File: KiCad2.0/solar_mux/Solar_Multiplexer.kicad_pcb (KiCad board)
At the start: 2 copper layers, 229.4 x 213.5 mm, 34 parts, among them J1 Conn_01x14, J2 Conn_02x06_Odd_Even, J3 Conn_02x06_Odd_Even, U1 ASSR-1611, U10 ASSR-1611, U11 ASSR-1611, U12 ASSR-1611, U13 ASSR-1611, U14 ASSR-1611, U15 ASSR-1611, U16 ASSR-1611, U17 ASSR-1611, U2 ASSR-1611, U20 ASSR-1611, U21 ASSR-1611, U22 MCP23S17, U3 ASSR-1611, U4 ASSR-1611, U5 ASSR-1611, U6 ASSR-1611, U7 ASSR-1611

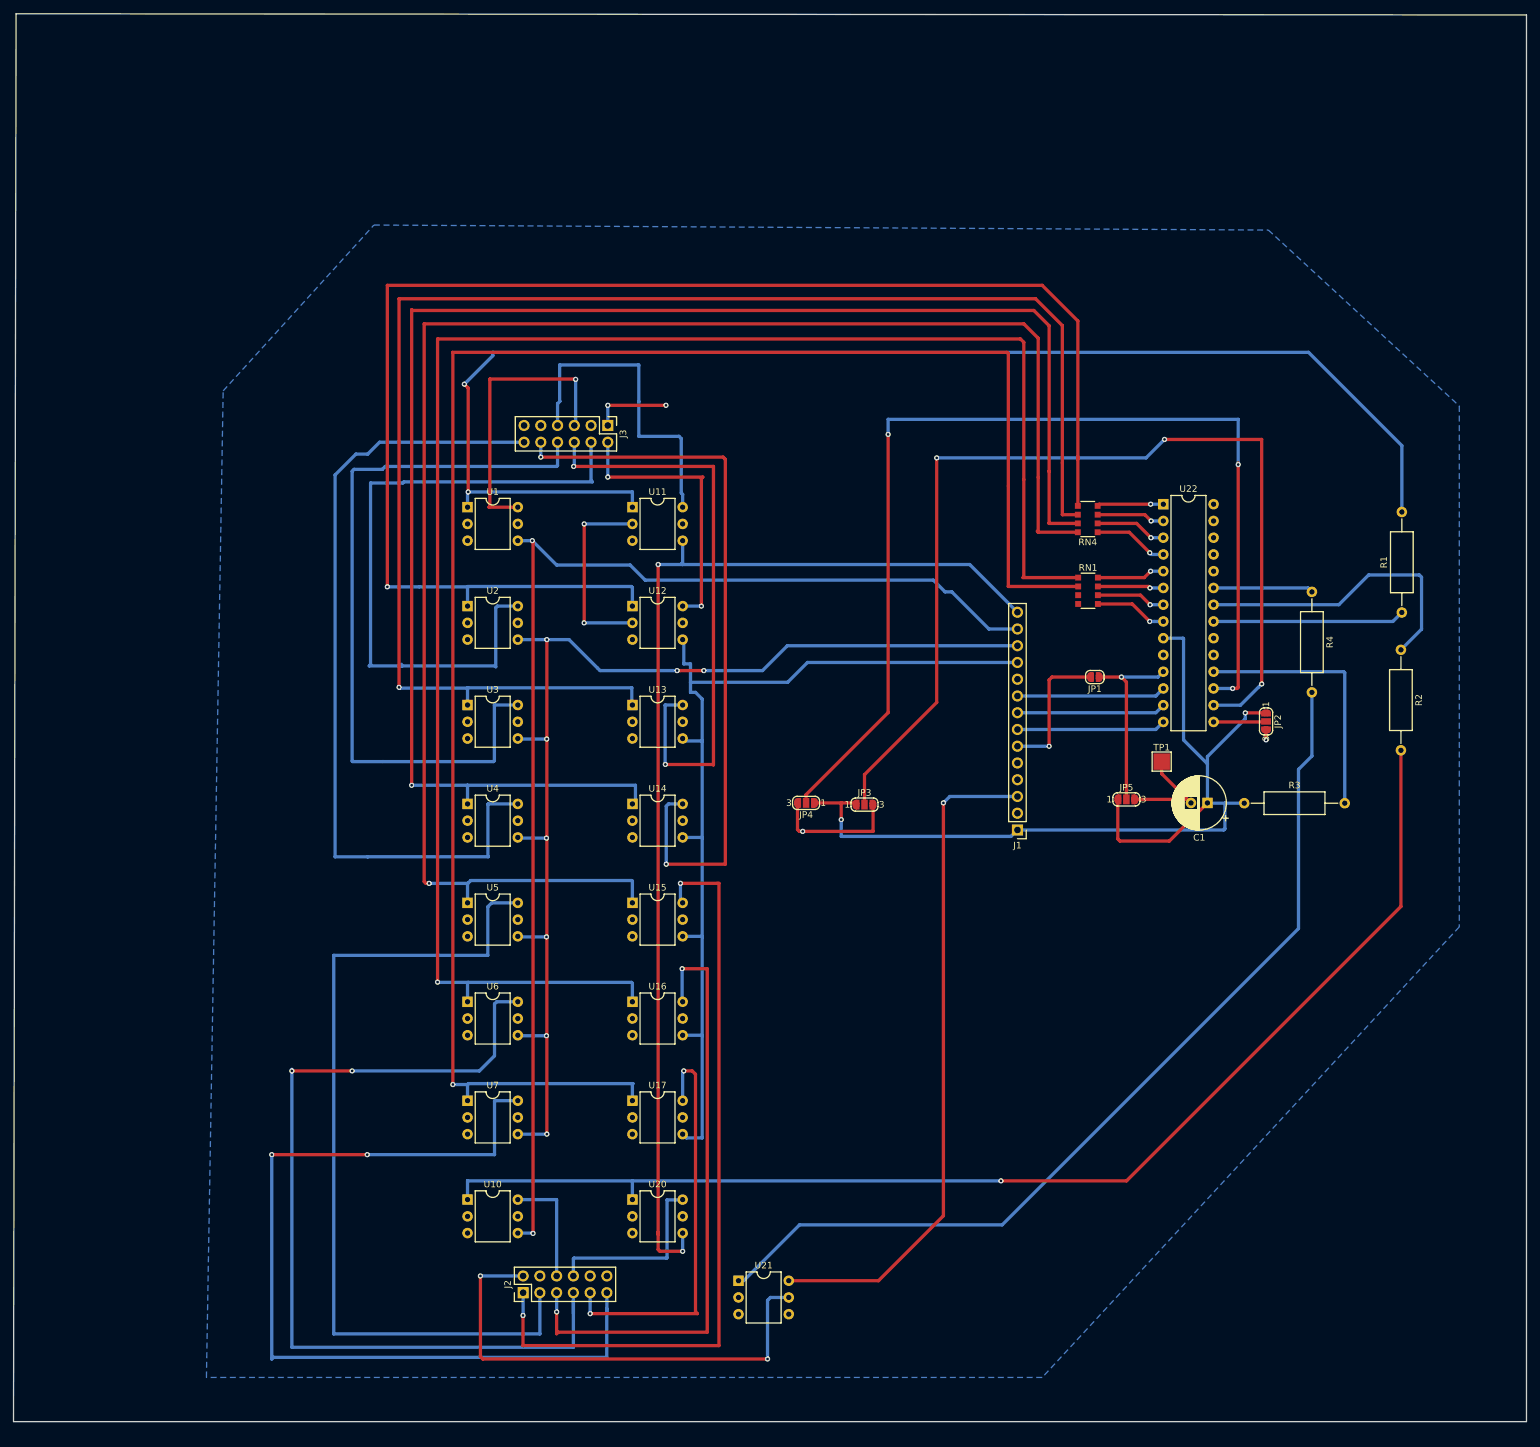
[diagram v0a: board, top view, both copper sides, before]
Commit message: Final Edits
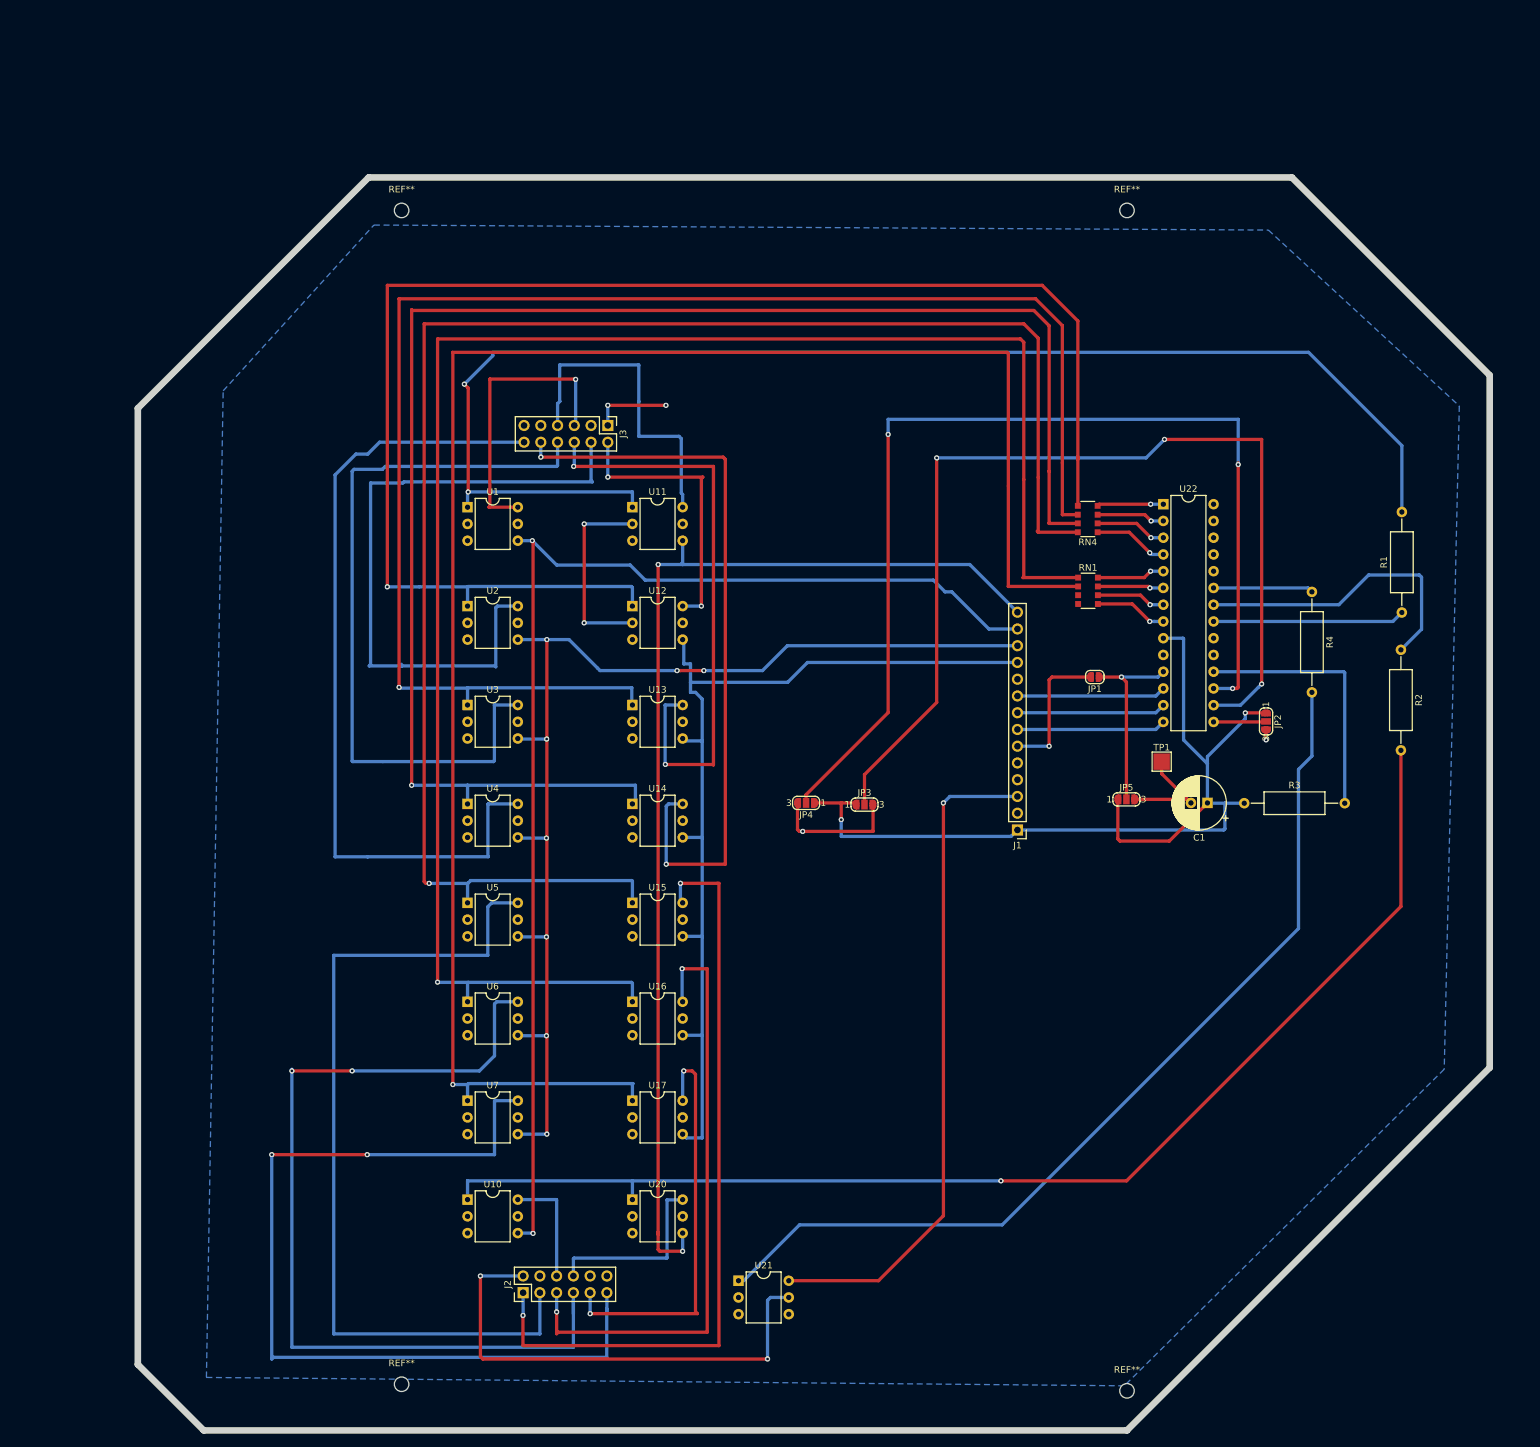
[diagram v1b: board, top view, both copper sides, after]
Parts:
- added REF**: MountingHole_2.2mm_M2, MountingHole:MountingHole_2.2mm_M2, F.Cu at (-310.0, 253.0)
- added REF**: MountingHole_2.2mm_M2, MountingHole:MountingHole_2.2mm_M2, F.Cu at (-200.0, 254.0)
- added REF**: MountingHole_2.2mm_M2, MountingHole:MountingHole_2.2mm_M2, F.Cu at (-200.0, 75.0)
- added REF**: MountingHole_2.2mm_M2, MountingHole:MountingHole_2.2mm_M2, F.Cu at (-310.0, 75.0)
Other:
- board size 229.4 x 213.5 mm -> 205 x 190 mm
